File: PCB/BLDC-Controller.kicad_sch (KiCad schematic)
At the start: 0 parts

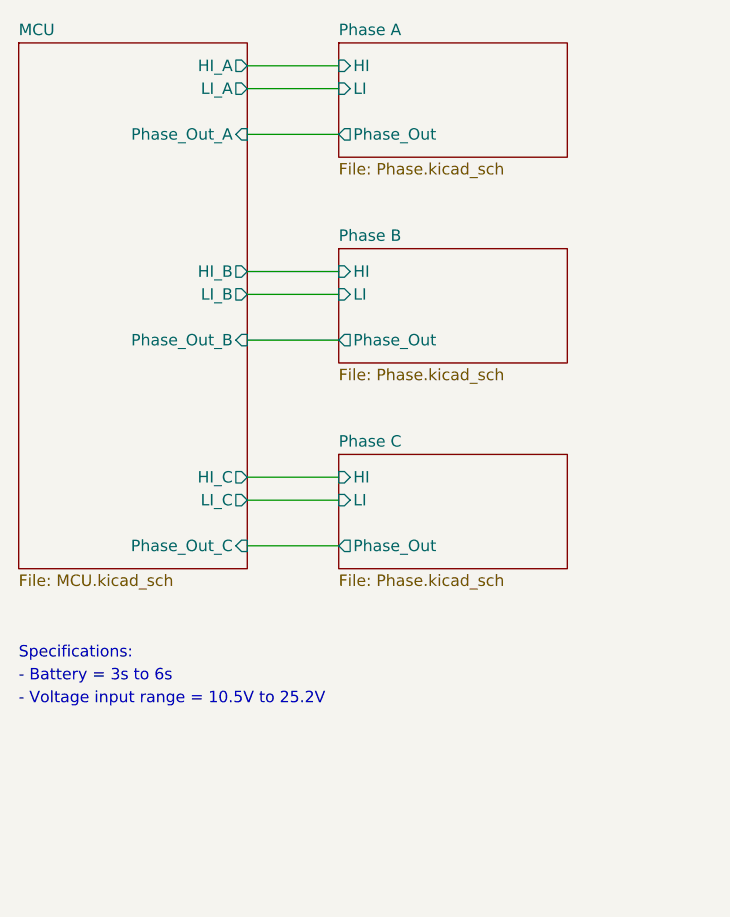
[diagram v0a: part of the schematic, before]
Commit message: V2 started
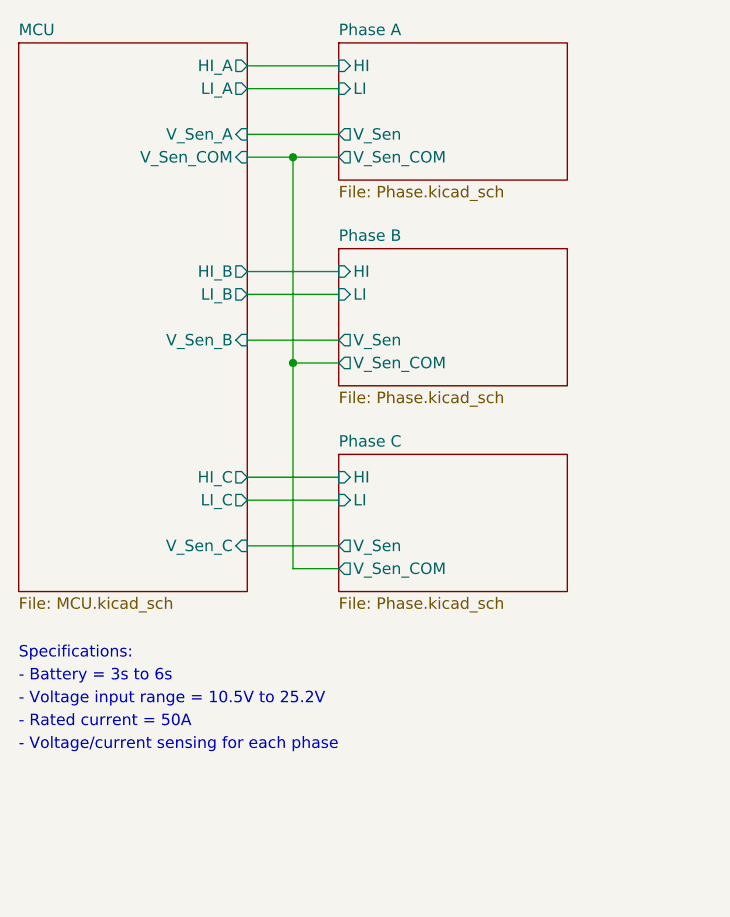
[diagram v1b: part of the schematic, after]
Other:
- sheet MCU ports: added V_Sen_A, V_Sen_B, V_Sen_C, V_Sen_COM; removed Phase_Out_A, Phase_Out_B, Phase_Out_C
- sheet Phase A ports: added V_Sen, V_Sen_COM; removed Phase_Out
- sheet Phase B ports: added V_Sen, V_Sen_COM; removed Phase_Out
- sheet Phase C ports: added V_Sen, V_Sen_COM; removed Phase_Out
- note added: "- Rated current = 50A"
- note added: "- Voltage/current sensing for each phase"
- company: Aria Tso -> (none)
- title: XE636 BLDC Motor Controller -> (none)
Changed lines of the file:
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@@
 (kicad_sch (version 20230121) (generator eeschema)
   (paper "A4")
-  (title_block
-    (title "XE636 BLDC Motor Controller")
-    (date "2024-03-09")
-    (rev "V1.0")
-    (company "Aria Tso")
+  (junction (at 50.8 35.56) (diameter 0) (color 0 0 0 0)
+  )
+  (junction (at 50.8 58.42) (diameter 0) (color 0 0 0 0)
+  )
+  (wire (pts (xy 45.72 33.02) (xy 55.88 33.02))
+    (stroke (width 0) (type default))
+  )
+  (wire (pts (xy 45.72 35.56) (xy 50.8 35.56))
+    (stroke (width 0) (type default))
+  )
+  (wire (pts (xy 45.72 78.74) (xy 55.88 78.74))
+    (stroke (width 0) (type default))
   )
   (wire (pts (xy 45.72 25.4) (xy 55.88 25.4))
     (stroke (width 0) (type default))
   )
-  (wire (pts (xy 45.72 33.02) (xy 55.88 33.02))
-    (stroke (width 0) (type default))
-  )
-  (wire (pts (xy 45.72 78.74) (xy 55.88 78.74))
+  (wire (pts (xy 45.72 55.88) (xy 55.88 55.88))
+    (stroke (width 0) (type default))
+  )
+  (wire (pts (xy 50.8 35.56) (xy 55.88 35.56))
+    (stroke (width 0) (type default))
+  )
+  (wire (pts (xy 50.8 58.42) (xy 50.8 81.28))
     (stroke (width 0) (type default))
   )
@@
     (stroke (width 0) (type default))
   )
+  (wire (pts (xy 55.88 58.42) (xy 50.8 58.42))
+    (stroke (width 0) (type default))
+  )
   (wire (pts (xy 45.72 27.94) (xy 55.88 27.94))
     (stroke (width 0) (type default))
   )
-  (wire (pts (xy 45.72 55.88) (xy 55.88 55.88))
-    (stroke (width 0) (type default))
-  )
   (wire (pts (xy 45.72 73.66) (xy 55.88 73.66))
     (stroke (width 0) (type default))
@@
     (stroke (width 0) (type default))
   )
+  (wire (pts (xy 50.8 81.28) (xy 55.88 81.28))
+    (stroke (width 0) (type default))
+  )
   (wire (pts (xy 45.72 48.26) (xy 55.88 48.26))
+    (stroke (width 0) (type default))
+  )
+  (wire (pts (xy 50.8 58.42) (xy 50.8 35.56))
     (stroke (width 0) (type default))
   )
@@
     )
   )
+  (text "- Voltage/current sensing for each phase" (at 20.32 101.6 0)
+    (effects (font (size 1.27 1.27)) (justify left bottom))
+  )
   (text "- Voltage input range = 10.5V to 25.2V" (at 20.32 96.52 0)
     (effects (font (size 1.27 1.27)) (justify left bottom))
@@
     (effects (font (size 1.27 1.27)) (justify left bottom))
   )
-  (sheet (at 55.88 22.86) (size 25.4 12.7) (fields_autoplaced)
+  (text "- Rated current = 50A" (at 20.32 99.06 0)
+    (effects (font (size 1.27 1.27)) (justify left bottom))
+  )
+  (sheet (at 55.88 22.86) (size 25.4 15.24) (fields_autoplaced)
     (stroke (width 0.1524) (type solid))
     (fill (color 0 0 0 0.0000))
@@
       (effects (font (size 1.27 1.27)) (justify left bottom))
     )
-    (property "Sheetfile" "Phase.kicad_sch" (at 55.88 36.1446 0)
+    (property "Sheetfile" "Phase.kicad_sch" (at 55.88 38.6846 0)
       (effects (font (size 1.27 1.27)) (justify left top))
-    )
-    (pin "Phase_Out" output (at 55.88 33.02 180)
-      (effects (font (size 1.27 1.27)) (justify left))
     )
     (pin "HI" input (at 55.88 25.4 180)
@@
     )
     (pin "LI" input (at 55.88 27.94 180)
+      (effects (font (size 1.27 1.27)) (justify left))
+    )
+    (pin "V_Sen_COM" output (at 55.88 35.56 180)
+      (effects (font (size 1.27 1.27)) (justify left))
+    )
+    (pin "V_Sen" output (at 55.88 33.02 180)
       (effects (font (size 1.27 1.27)) (justify left))
     )
@@
     )
   )
-  (sheet (at 55.88 45.72) (size 25.4 12.7) (fields_autoplaced)
+  (sheet (at 55.88 45.72) (size 25.4 15.24) (fields_autoplaced)
     (stroke (width 0.1524) (type solid))
     (fill (color 0 0 0 0.0000))
@@
       (effects (font (size 1.27 1.27)) (justify left bottom))
     )
-    (property "Sheetfile" "Phase.kicad_sch" (at 55.88 59.0046 0)
+    (property "Sheetfile" "Phase.kicad_sch" (at 55.88 61.5446 0)
       (effects (font (size 1.27 1.27)) (justify left top))
-    )
-    (pin "Phase_Out" output (at 55.88 55.88 180)
-      (effects (font (size 1.27 1.27)) (justify left))
     )
     (pin "HI" input (at 55.88 48.26 180)
@@
     )
     (pin "LI" input (at 55.88 50.8 180)
+      (effects (font (size 1.27 1.27)) (justify left))
+    )
+    (pin "V_Sen_COM" output (at 55.88 58.42 180)
+      (effects (font (size 1.27 1.27)) (justify left))
+    )
+    (pin "V_Sen" output (at 55.88 55.88 180)
       (effects (font (size 1.27 1.27)) (justify left))
     )
@@
     )
   )
-  (sheet (at 55.88 68.58) (size 25.4 12.7) (fields_autoplaced)
+  (sheet (at 55.88 68.58) (size 25.4 15.24) (fields_autoplaced)
     (stroke (width 0.1524) (type solid))
     (fill (color 0 0 0 0.0000))
@@
       (effects (font (size 1.27 1.27)) (justify left bottom))
     )
-    (property "Sheetfile" "Phase.kicad_sch" (at 55.88 81.8646 0)
+    (property "Sheetfile" "Phase.kicad_sch" (at 55.88 84.4046 0)
       (effects (font (size 1.27 1.27)) (justify left top))
-    )
-    (pin "Phase_Out" output (at 55.88 78.74 180)
-      (effects (font (size 1.27 1.27)) (justify left))
     )
     (pin "HI" input (at 55.88 71.12 180)
@@
     )
     (pin "LI" input (at 55.88 73.66 180)
+      (effects (font (size 1.27 1.27)) (justify left))
+    )
+    (pin "V_Sen_COM" output (at 55.88 81.28 180)
+      (effects (font (size 1.27 1.27)) (justify left))
+    )
+    (pin "V_Sen" output (at 55.88 78.74 180)
       (effects (font (size 1.27 1.27)) (justify left))
     )
@@
     )
   )
-  (sheet (at 20.32 22.86) (size 25.4 58.42) (fields_autoplaced)
+  (sheet (at 20.32 22.86) (size 25.4 60.96) (fields_autoplaced)
     (stroke (width 0.1524) (type solid))
     (fill (color 0 0 0 0.0000))
@@
       (effects (font (size 1.27 1.27)) (justify left bottom))
     )
-    (property "Sheetfile" "MCU.kicad_sch" (at 20.32 81.8646 0)
+    (property "Sheetfile" "MCU.kicad_sch" (at 20.32 84.4046 0)
       (effects (font (size 1.27 1.27)) (justify left top))
     )
@@
       (effects (font (size 1.27 1.27)) (justify right))
     )
-    (pin "Phase_Out_C" input (at 45.72 78.74 0)
+    (pin "V_Sen_COM" input (at 45.72 35.56 0)
       (effects (font (size 1.27 1.27)) (justify right))
     )
-    (pin "Phase_Out_B" input (at 45.72 55.88 0)
+    (pin "V_Sen_B" input (at 45.72 55.88 0)
       (effects (font (size 1.27 1.27)) (justify right))
     )
-    (pin "Phase_Out_A" input (at 45.72 33.02 0)
+    (pin "V_Sen_A" input (at 45.72 33.02 0)
       (effects (font (size 1.27 1.27)) (justify right))
     )
+    (pin "V_Sen_C" input (at 45.72 78.74 0)
+      (effects (font (size 1.27 1.27)) (justify right))
+    )
